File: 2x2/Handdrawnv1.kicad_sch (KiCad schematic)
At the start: 31 parts, among them J2 USB_B_Mini, K1 KEYSW, K2 KEYSW, K3 KEYSW, K4 KEYSW, SW1 SW_PUSH, U1 ATMEGA32U4, Y2 Crystal_GND24_Small

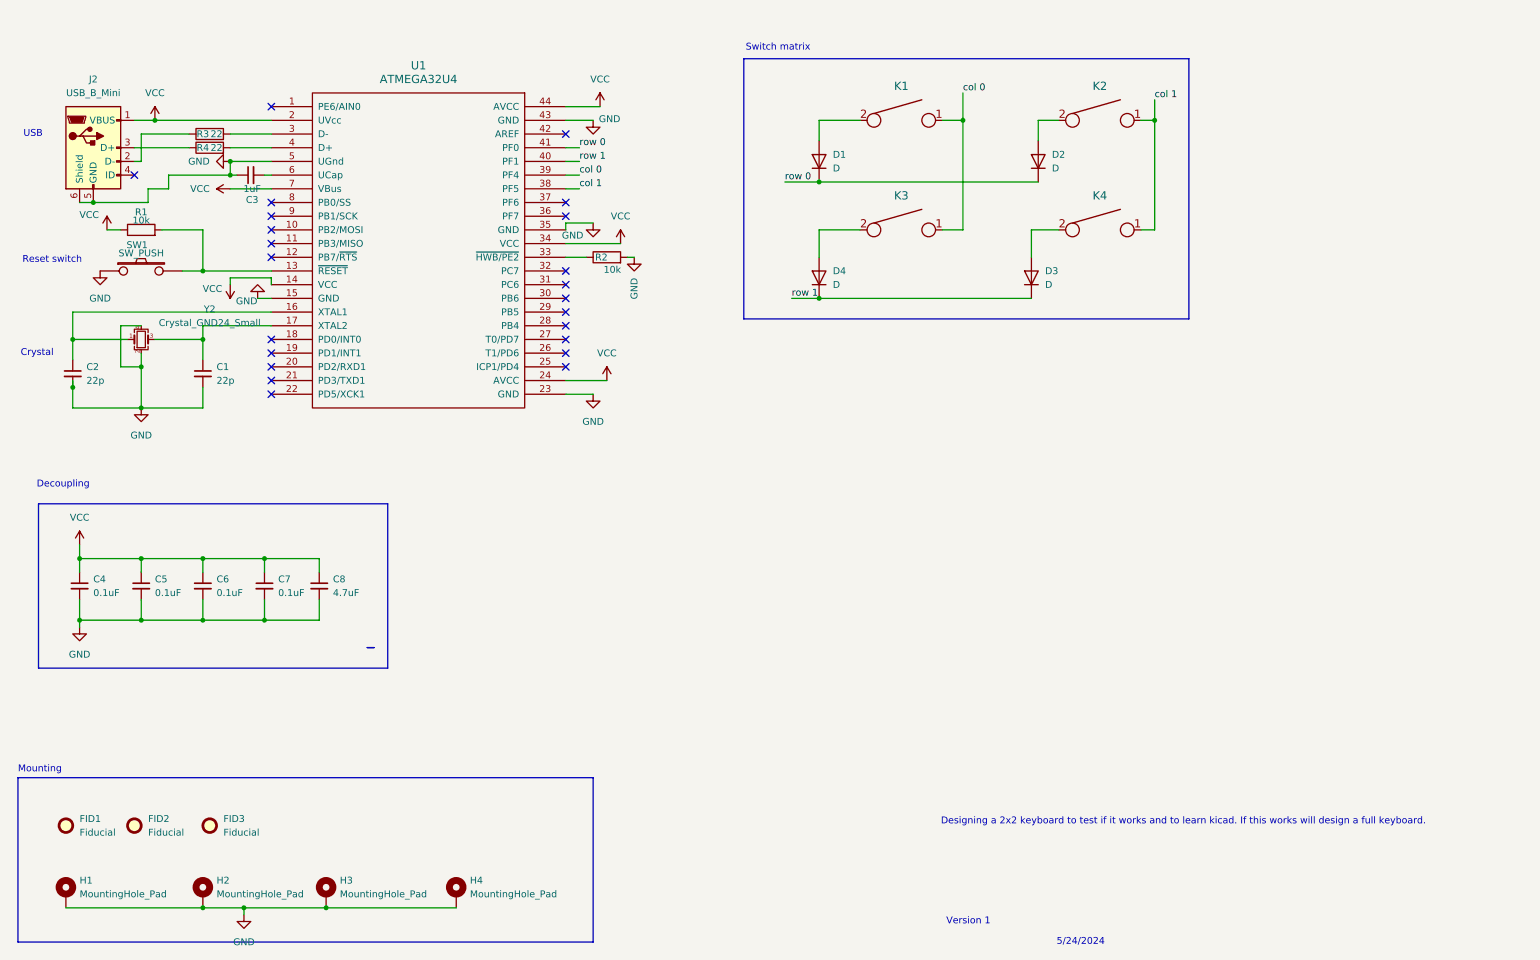
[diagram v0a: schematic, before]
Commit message: almost finished the 2x2, will be working on the 65 now
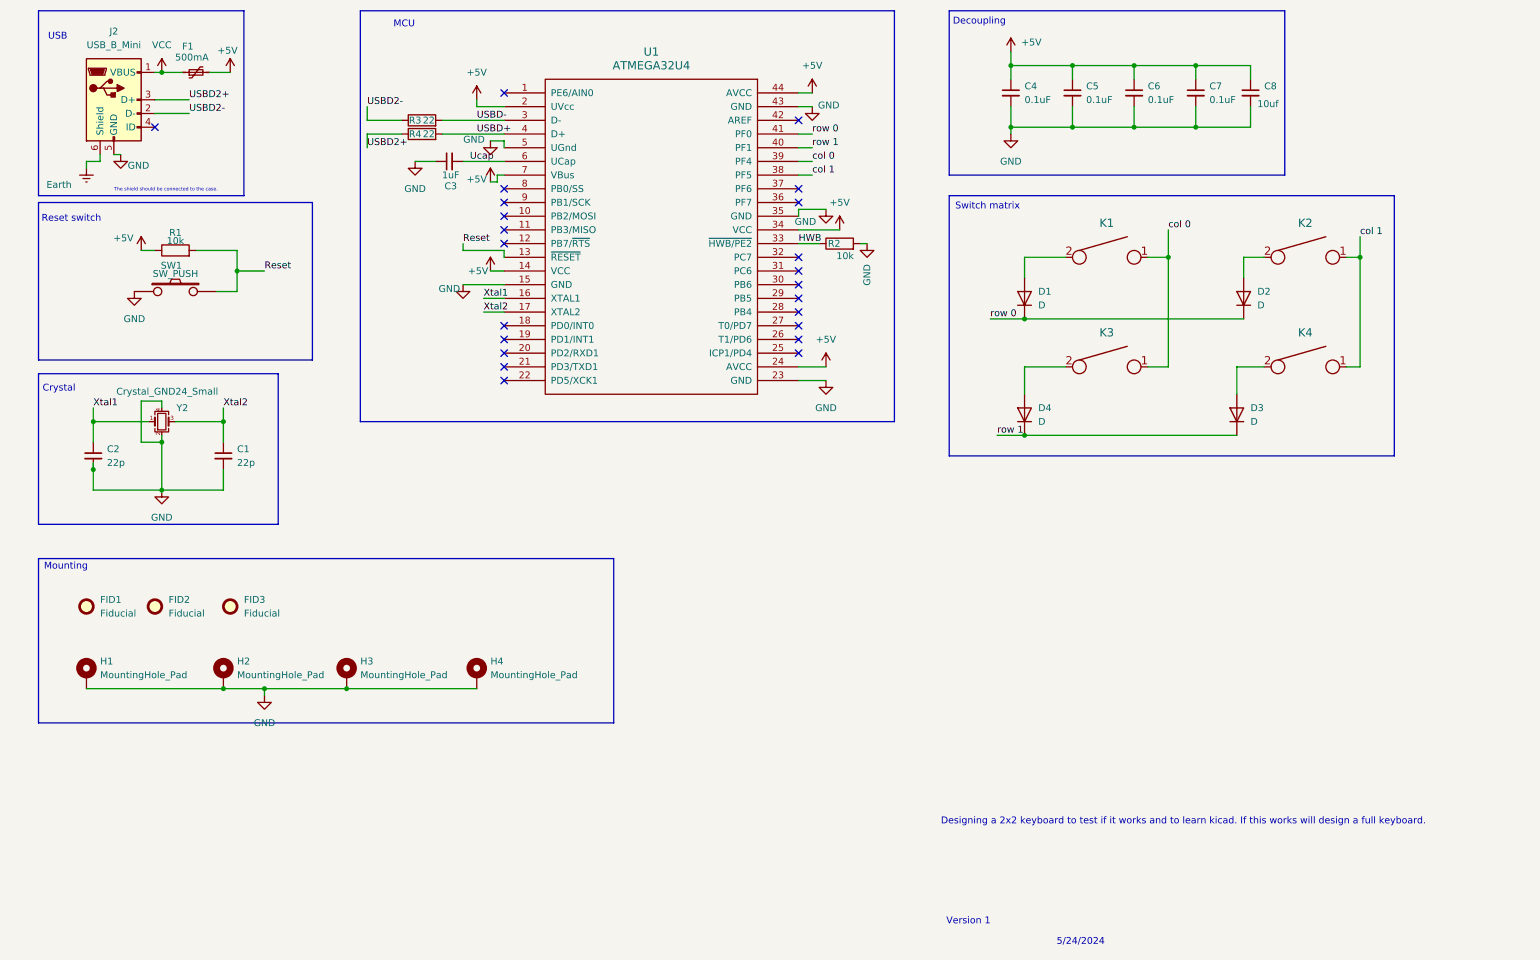
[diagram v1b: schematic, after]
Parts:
- added F1: 500mA, Fuse:Fuse_1206_3216Metric_Pad1.42x1.75mm_HandSolder, symbol Device:Polyfuse_Small
- C8: value 4.7uF -> 10uf
- SW1: footprint Button_Switch_SMD:SW_SPST_TL3342 -> Button_Switch_SMD:SW_SPST_SKQG_WithStem
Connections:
- net GND: no longer J2.6 (Shield)
- net VCC: now also F1.1; no longer C4.1, C5.1, C6.1, C7.1, C8.1, R1.1, U1.14 (VCC), U1.2 (UVcc), U1.24 (AVCC), U1.34 (VCC), U1.44 (AVCC), U1.7 (VBus)
- net Xtal1: now reaches C2.1, U1.16 (XTAL1), Y2.1
- net USBD2-: now reaches J2.2 (D-), R3.1
- net USBD-: now reaches R3.2, U1.3 (D-)
- net USBD2+: now reaches J2.3 (D+), R4.1
- net USBD+: now reaches R4.2, U1.4 (D+)
- net Reset: now reaches R1.2, SW1.2, U1.13 (~{RESET})
- net Ucap: now reaches C3.2, U1.6 (UCap)
- net HWB: now reaches R2.1, U1.33 (~{HWB/PE2})
- net Xtal2: now reaches C1.1, U1.17 (XTAL2), Y2.3
- new net +5V: C4.1, C5.1, C6.1, C7.1, C8.1, F1.2, R1.1, U1.14 (VCC), U1.2 (UVcc), U1.24 (AVCC), U1.34 (VCC), U1.44 (AVCC), U1.7 (VBus)
- new net Earth: J2.6 (Shield)
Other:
- note added: "MCU"
- note added: "The shield should be connected to the case."
- moved on the sheet: C1, C2, C3, C4, C5, C6, C7, C8, D1, D2, D3, D4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
